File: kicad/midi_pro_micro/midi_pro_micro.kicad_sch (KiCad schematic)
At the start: 28 parts, among them J1 DIN-5_180degree, J2 DIN-5_180degree, J3 Conn_01x12, J4 Conn_01x16_Pin, J6 Conn_01x04, U1 ProMicro, U2 AT25xxx, U3 6N138

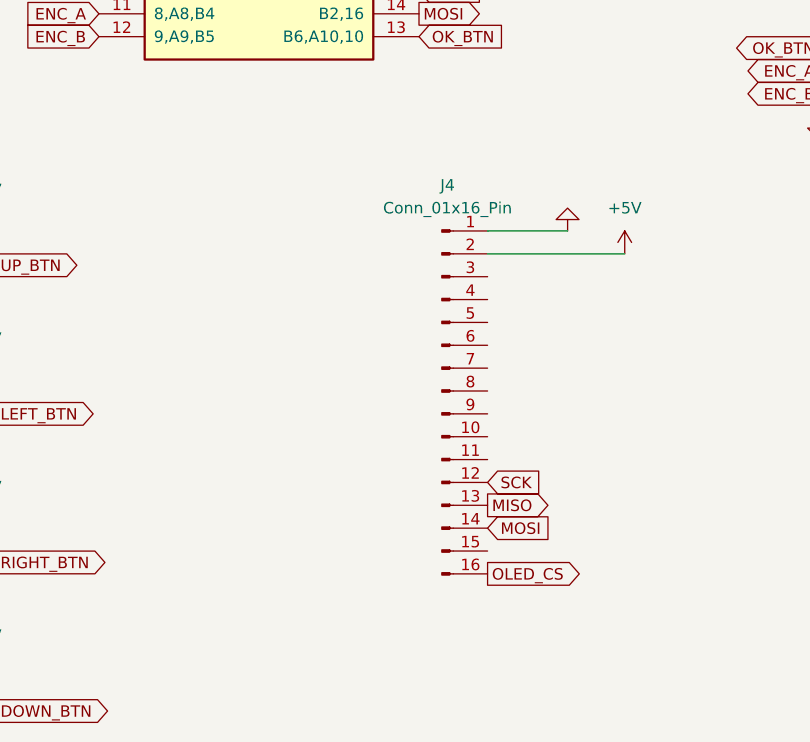
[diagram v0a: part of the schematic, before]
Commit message: Basic layout ready
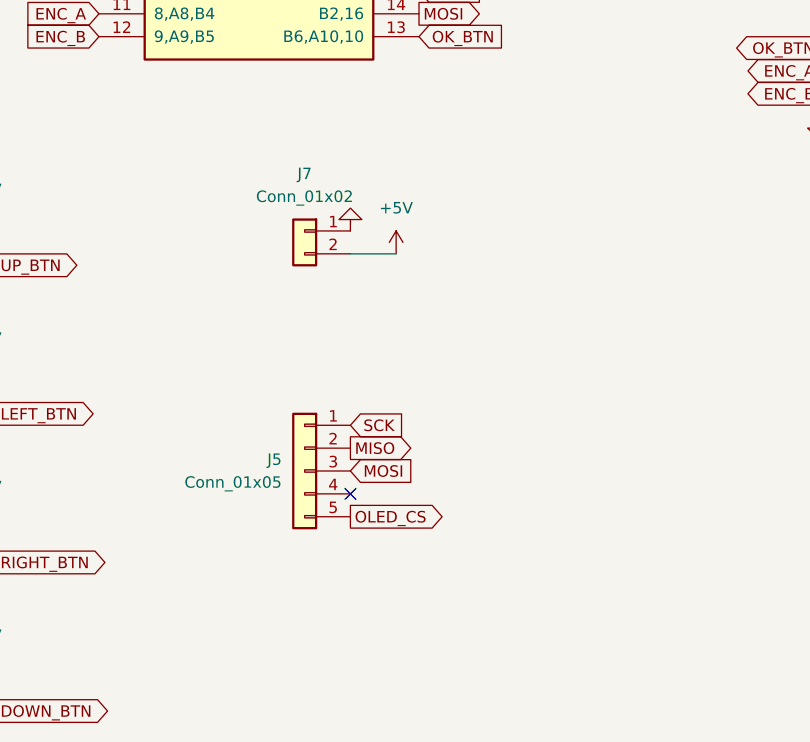
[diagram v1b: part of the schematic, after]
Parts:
- removed J4: Conn_01x16_Pin, Connector_PinHeader_2.54mm:PinHeader_1x16_P2.54mm_Vertical, symbol Connector:Conn_01x16_Pin
- added J5: Conn_01x05, Connector_JST:JST_PH_B5B-PH-K_1x05_P2.00mm_Vertical, symbol Connector_Generic:Conn_01x05
- added J7: Conn_01x02, Connector_JST:JST_PH_B2B-PH-K_1x02_P2.00mm_Vertical, symbol Connector_Generic:Conn_01x02
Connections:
- net +5V: now also J7.2 (Pin_2)
- net GND: now also J7.1 (Pin_1)
- net MISO: now also J5.2 (Pin_2)
- net MOSI: now also J5.3 (Pin_3)
- net OLED_CS: now also J5.5 (Pin_5)
- net SCK: now also J5.1 (Pin_1)
- no-connect marks 0 -> 1

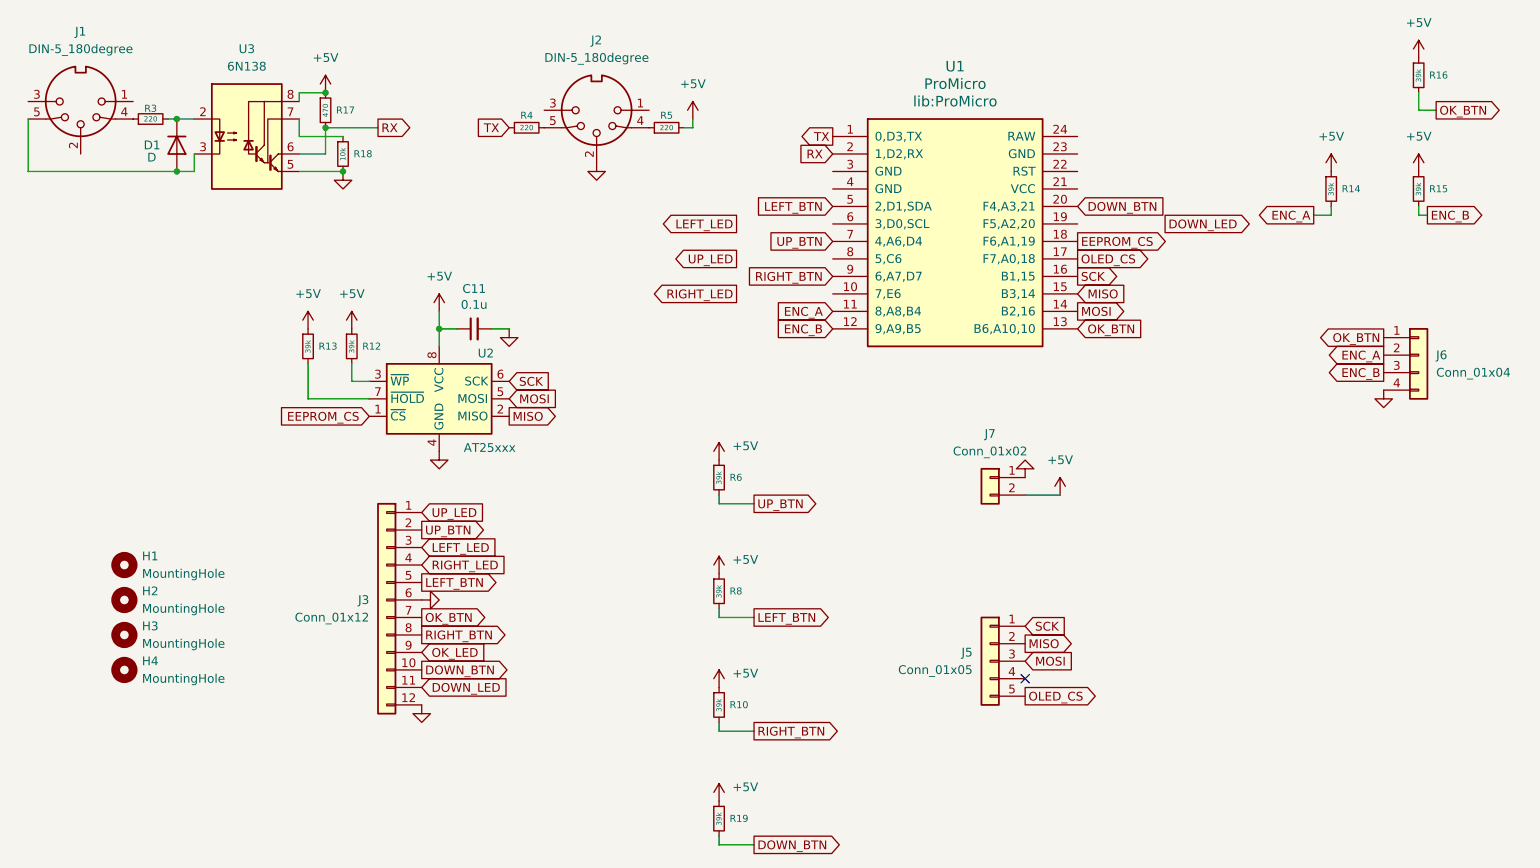
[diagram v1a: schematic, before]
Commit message: Start PCB trace
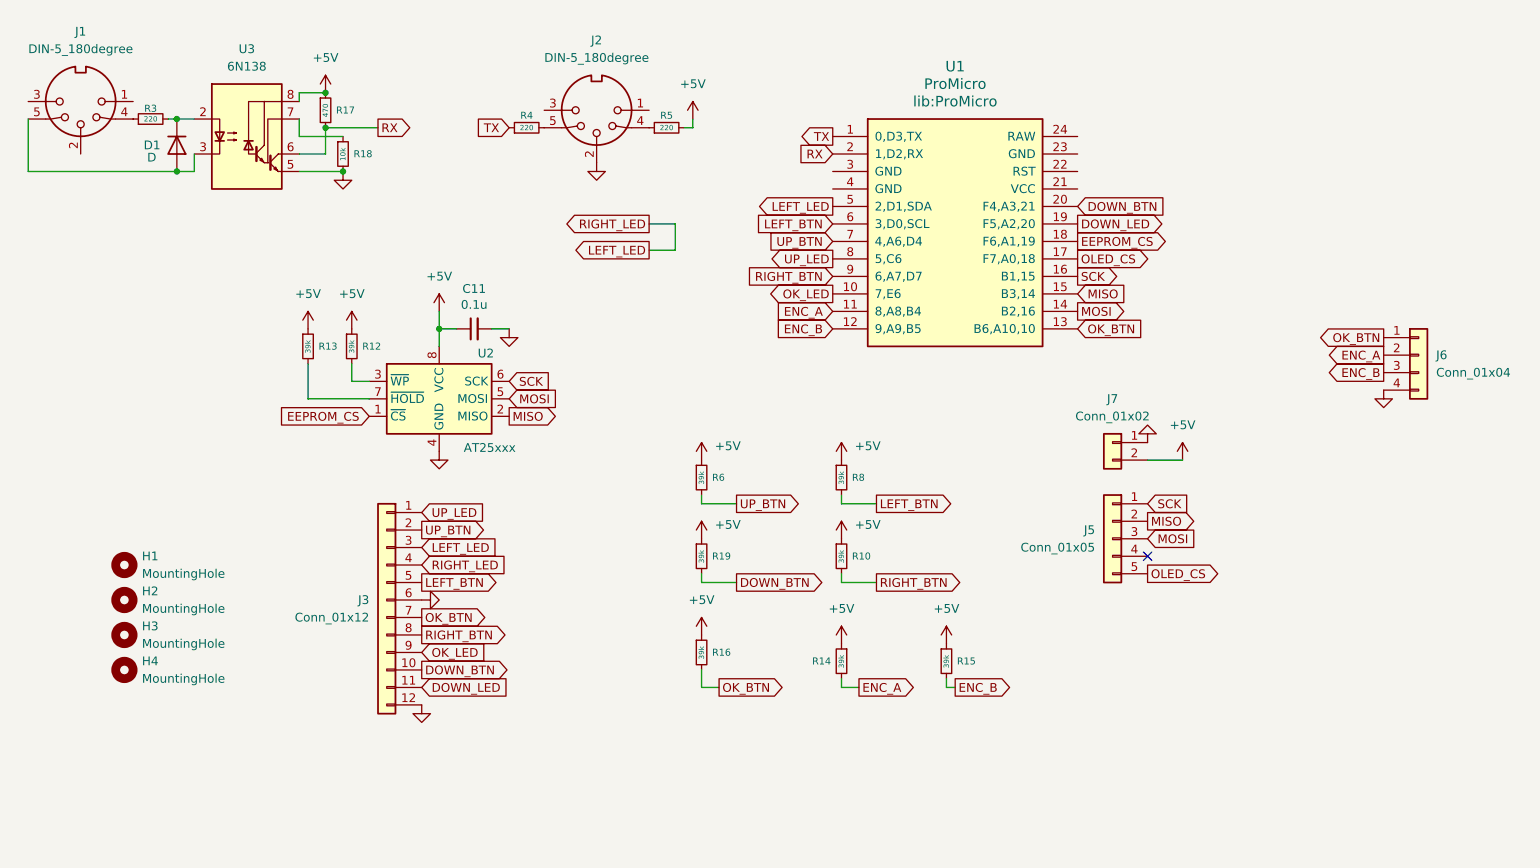
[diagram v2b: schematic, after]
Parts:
- D1: footprint (none) -> Diode_SMD:D_SOD-323_HandSoldering
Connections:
- net RIGHT_LED is gone; now on net LEFT_LED: J3.4 (Pin_4)
- net DOWN_LED: now also U1.19 (F5,A2,20)
- net LEFT_BTN: now also U1.6 (3,D0,SCL); no longer U1.5 (2,D1,SDA)
- net LEFT_LED: now also U1.5 (2,D1,SDA)
- net OK_LED: now also U1.10 (7,E6)
- net UP_LED: now also U1.8 (5,C6)
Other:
- moved on the sheet: J5, J7, R10, R14, R15, R16, R19, R6, R8

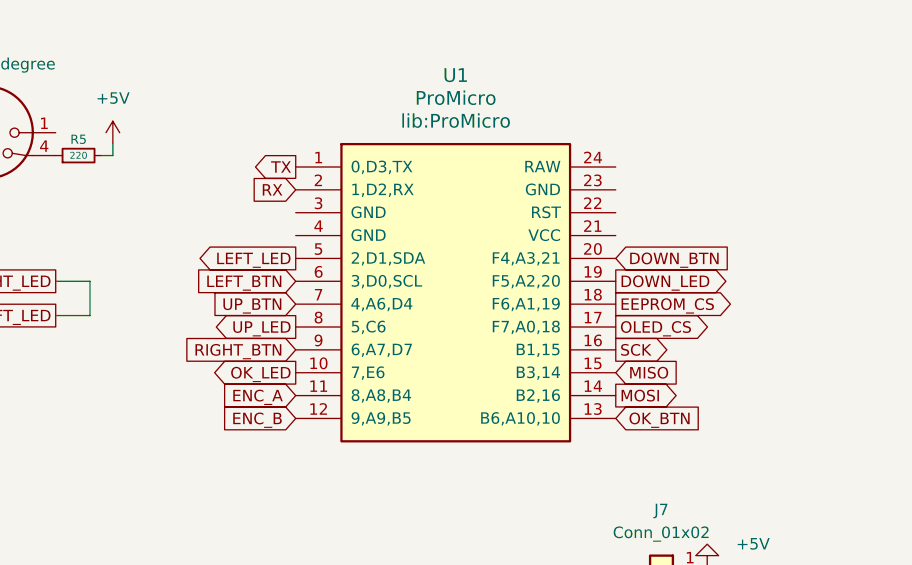
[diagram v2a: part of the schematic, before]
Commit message: PCB trace finished
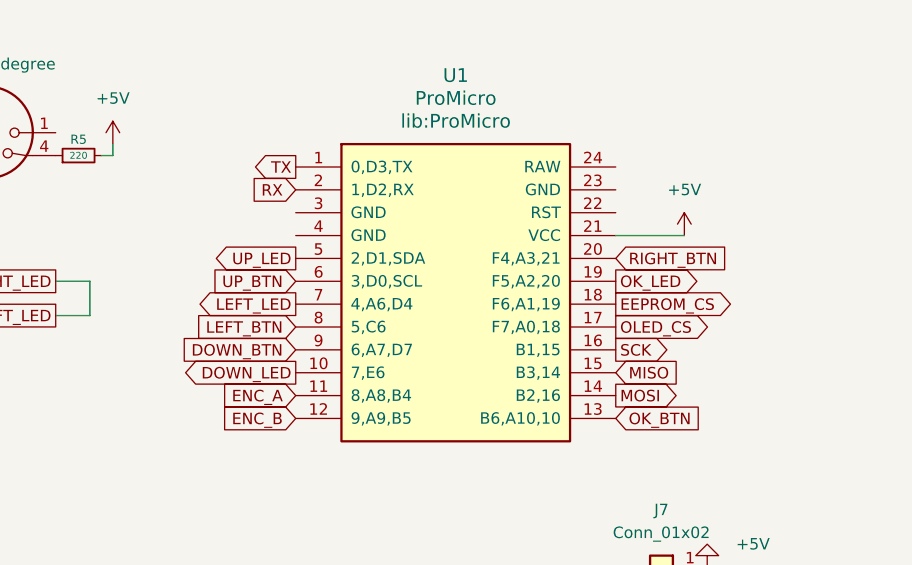
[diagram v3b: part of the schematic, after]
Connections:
- net +5V: now also U1.21 (VCC)
- net DOWN_BTN: now also U1.9 (6,A7,D7); no longer U1.20 (F4,A3,21)
- net DOWN_LED: now also U1.10 (7,E6); no longer U1.19 (F5,A2,20)
- net LEFT_BTN: now also U1.8 (5,C6); no longer U1.6 (3,D0,SCL)
- net LEFT_LED: now also U1.7 (4,A6,D4); no longer U1.5 (2,D1,SDA)
- net OK_LED: now also U1.19 (F5,A2,20); no longer U1.10 (7,E6)
- net RIGHT_BTN: now also U1.20 (F4,A3,21); no longer U1.9 (6,A7,D7)
- net UP_BTN: now also U1.6 (3,D0,SCL); no longer U1.7 (4,A6,D4)
- net UP_LED: now also U1.5 (2,D1,SDA); no longer U1.8 (5,C6)
